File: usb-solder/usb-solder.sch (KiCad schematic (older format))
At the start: 303 parts, among them J1 USB_B_Micro, J10 USB_B_Micro, J11 USB_B_Micro, J12 USB_B_Micro, J13 USB_B_Micro, J14 USB_B_Micro, J15 USB_B_Micro, J16 USB_B_Micro, J17 USB_B_Micro, J18 USB_B_Micro, J19 USB_B_Micro, J2 USB_B_Micro, J20 USB_B_Micro, J21 USB_B_Micro, J22 USB_B_Micro, J23 USB_A, J24 Conn_01x02_Male, J25 Barrel_Jack_Switch, J26 USB_B_Micro, J27 Conn_01x07_Male, J3 USB_B_Micro, J4 USB_B_Micro, J5 USB_B_Micro, J6 USB_B_Micro, J7 USB_B_Micro, J8 USB_B_Micro, J9 USB_B_Micro, SW1 SW_SPDT, U1 555, U2 74HC164, U3 4072, U4 74AHC1G04, U5 AP1117-33

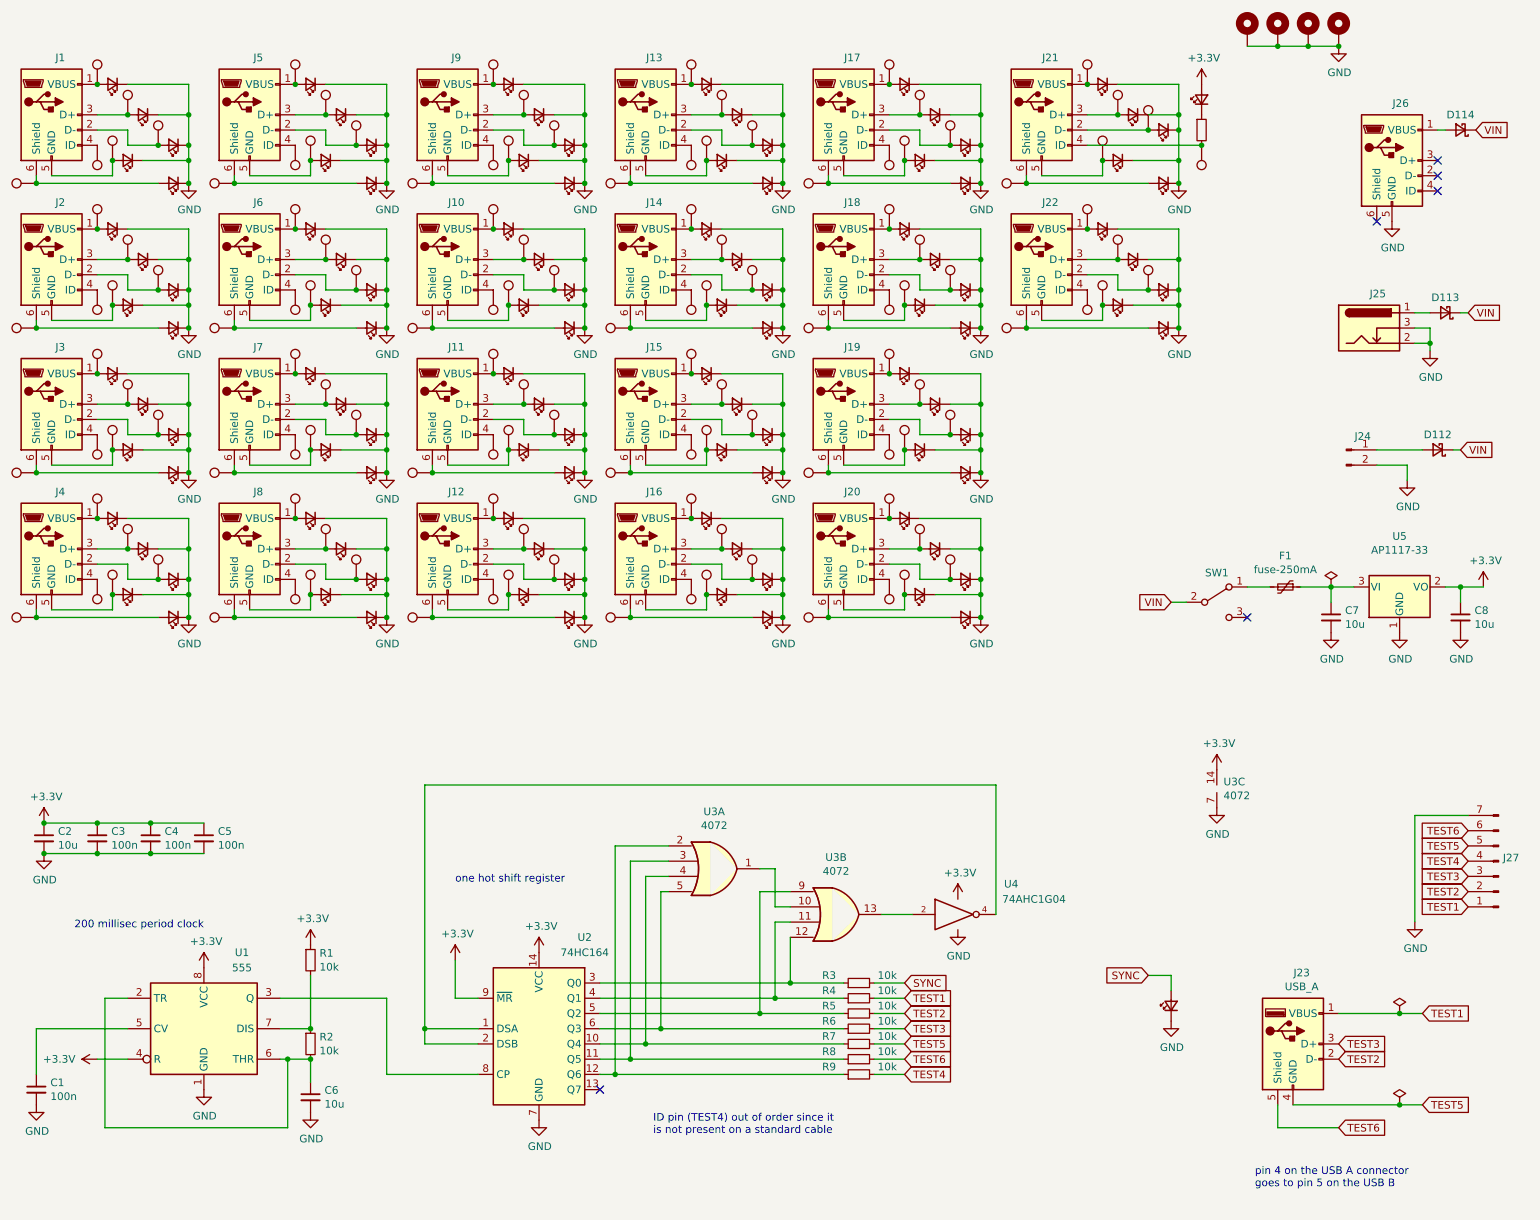
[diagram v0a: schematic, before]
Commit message: id
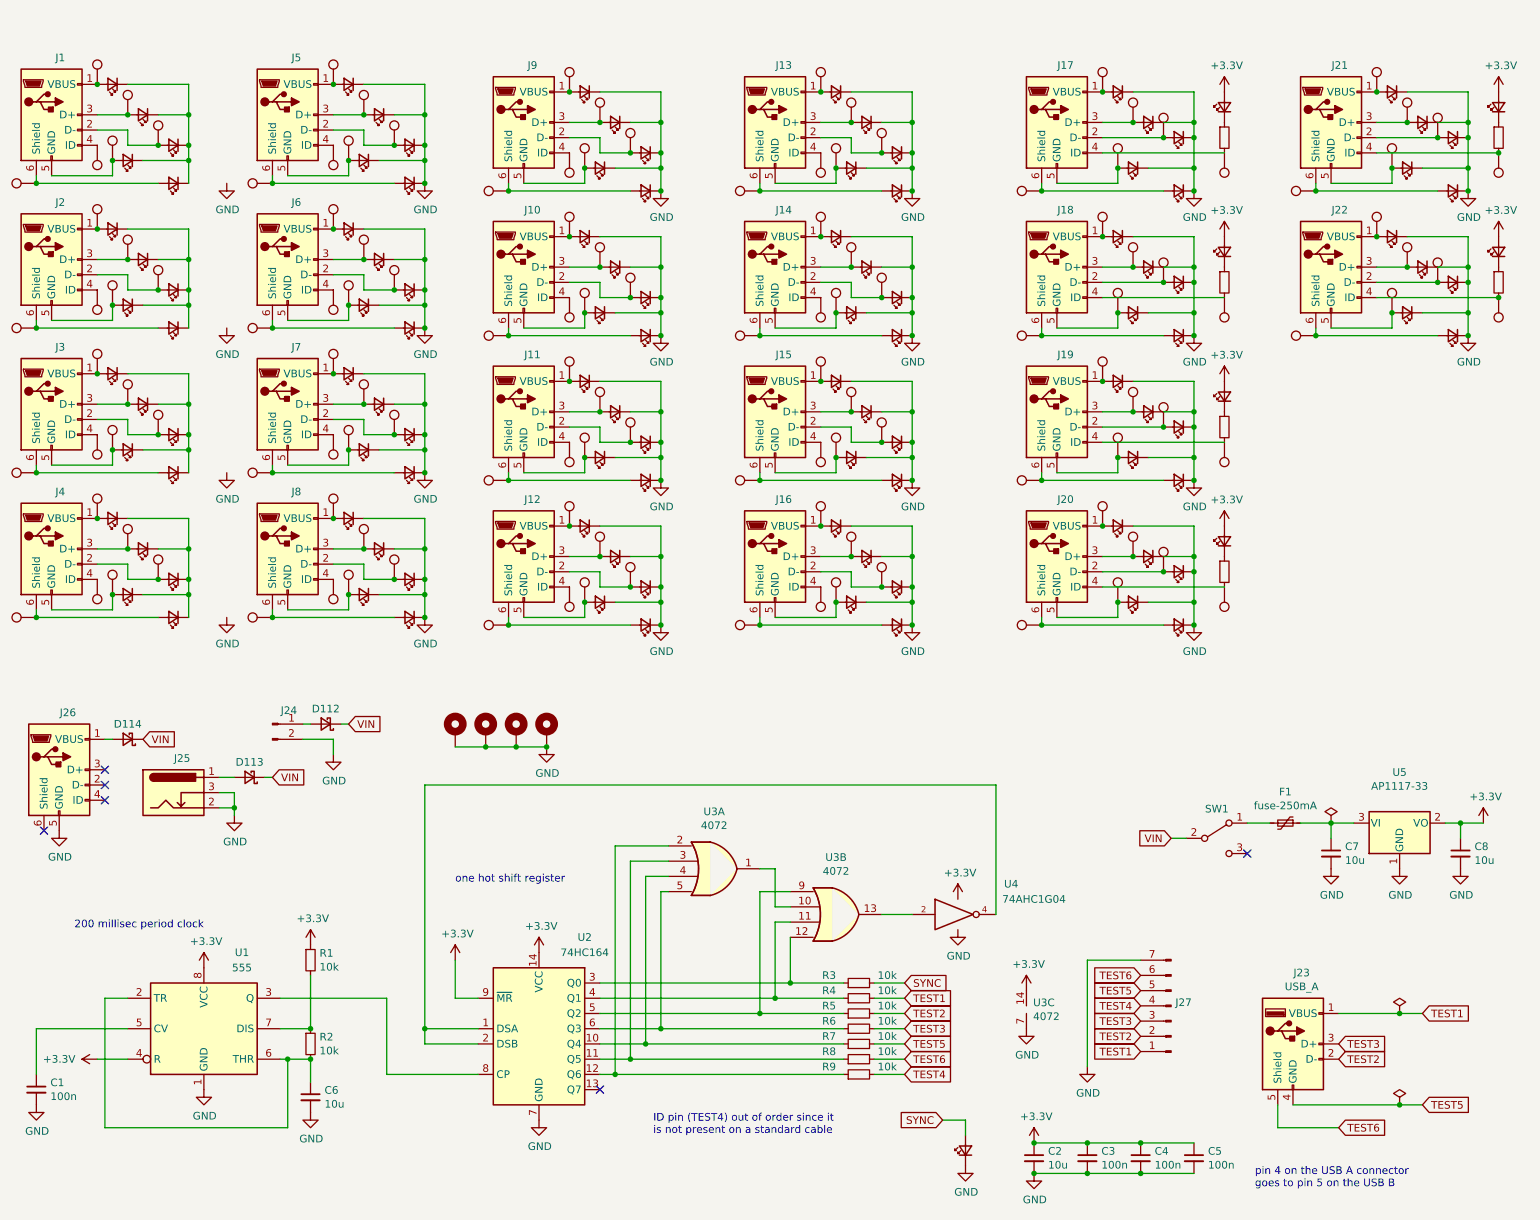
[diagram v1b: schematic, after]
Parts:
- added D116, D117, D118, D119, D120: ledred, LED_SMD:LED_0603_1608Metric, symbol pace:ledred
- added R11, R12, R13, R14, R15: 10k, Resistor_SMD:R_0402_1005Metric, symbol pace:10k
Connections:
- net +3V3: now also D116.2 (A), D117.2 (A), D118.2 (A), D119.2 (A), D120.2 (A)
- net GND: no longer D1.1 (K), D10.1 (K), D11.1 (K), D12.1 (K), D13.1 (K), D14.1 (K), D15.1 (K), D16.1 (K), D17.1 (K), D18.1 (K), D19.1 (K), D2.1 (K), D20.1 (K), D3.1 (K), D4.1 (K), D5.1 (K), D6.1 (K), D7.1 (K), D8.1 (K), D9.1 (K)
- net at J17.4 (ID), TP102.1: now also R11.2
- net at J18.4 (ID), TP104.1: now also R12.2
- net at J19.4 (ID), TP106.1: now also R13.2
- net at J20.4 (ID), TP108.1: now also R14.2
- net at J22.4 (ID), TP126.1: now also R15.2
- new net: D1.1 (K), D13.1 (K), D14.1 (K), D5.1 (K), D9.1 (K)
- new net: D10.1 (K), D15.1 (K), D16.1 (K), D2.1 (K), D6.1 (K)
- new net: D11.1 (K), D17.1 (K), D18.1 (K), D3.1 (K), D7.1 (K)
- new net: D12.1 (K), D19.1 (K), D20.1 (K), D4.1 (K), D8.1 (K)
- new net: D120.1 (K), R15.1
- new net: D116.1 (K), R11.1
- new net: D117.1 (K), R12.1
- new net: D118.1 (K), R13.1
- new net: D119.1 (K), R14.1
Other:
- moved on the sheet: C2, C3, C4, C5, C7, C8, D112, D113, D114, F1, J10, J11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

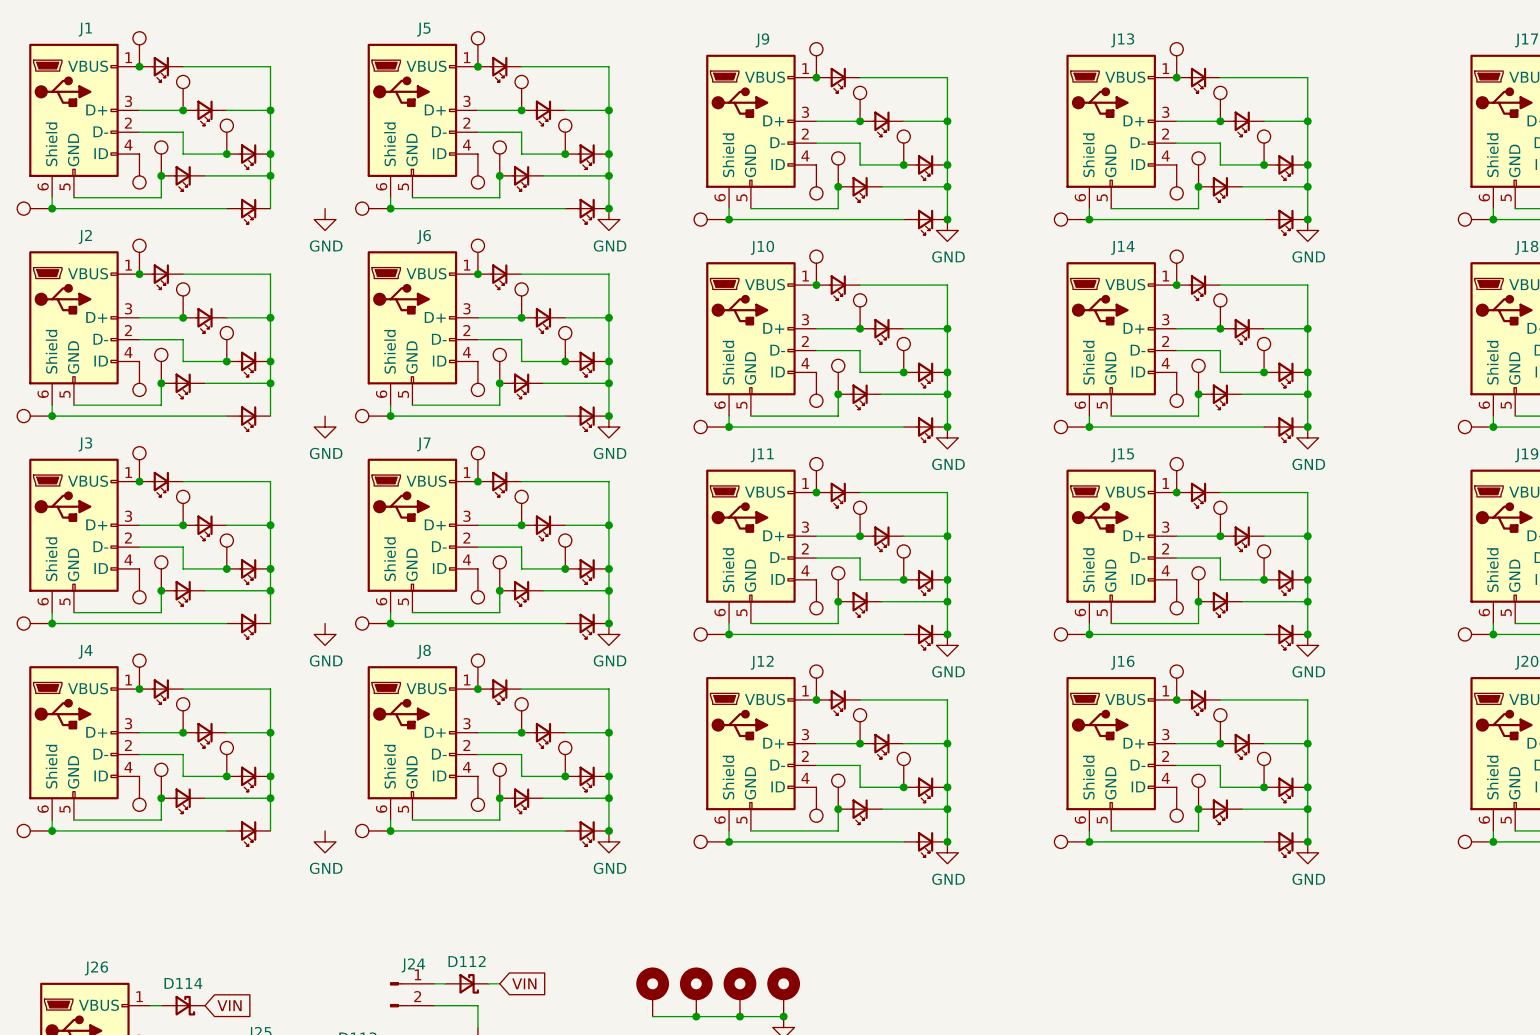
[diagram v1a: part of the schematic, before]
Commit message: id
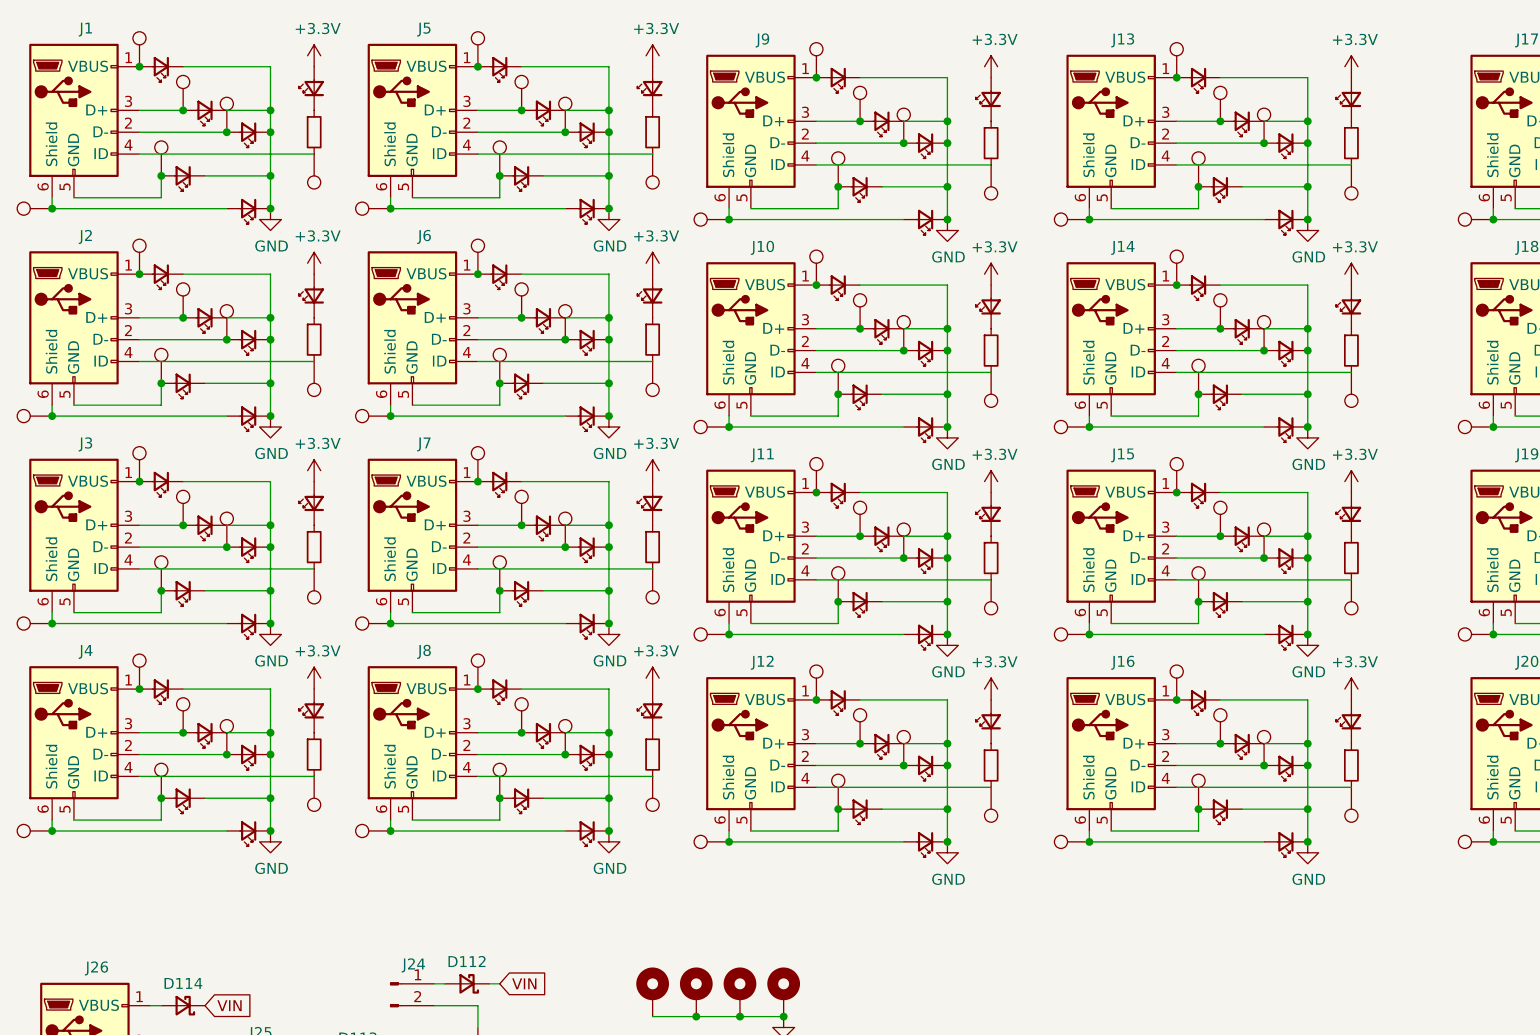
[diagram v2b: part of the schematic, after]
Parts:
- added D121, D122, D123, D124, D125, D126, D127, D128, D129, D130, D131, D132, D133, D134, D135, D136: ledred, LED_SMD:LED_0603_1608Metric, symbol pace:ledred
- added R16, R17, R18, R19, R20, R21, R22, R23, R24, R25, R26, R27, R28, R29, R30, R31: 10k, Resistor_SMD:R_0402_1005Metric, symbol pace:10k
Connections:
- net +3V3: now also D121.2 (A), D122.2 (A), D123.2 (A), D124.2 (A), D125.2 (A), D126.2 (A), D127.2 (A), D128.2 (A), D129.2 (A), D130.2 (A), D131.2 (A), D132.2 (A), D133.2 (A), D134.2 (A), D135.2 (A), D136.2 (A)
- net GND: now also D1.1 (K), D10.1 (K), D11.1 (K), D12.1 (K), D13.1 (K), D14.1 (K), D15.1 (K), D16.1 (K), D17.1 (K), D18.1 (K), D19.1 (K), D2.1 (K), D20.1 (K), D3.1 (K), D4.1 (K), D5.1 (K), D6.1 (K), D7.1 (K), D8.1 (K), D9.1 (K)
- net at J1.4 (ID), TP6.1: now also R16.2
- net at J2.4 (ID), TP8.1: now also R17.2
- net at J3.4 (ID), TP10.1: now also R18.2
- net at J4.4 (ID), TP12.1: now also R19.2
- net at J5.4 (ID), TP30.1: now also R20.2
- net at J6.4 (ID), TP32.1: now also R21.2
- net at J7.4 (ID), TP34.1: now also R22.2
- net at J8.4 (ID), TP36.1: now also R23.2
- net at J9.4 (ID), TP54.1: now also R24.2
- net at J10.4 (ID), TP56.1: now also R25.2
- net at J11.4 (ID), TP58.1: now also R26.2
- net at J12.4 (ID), TP60.1: now also R27.2
- net at J13.4 (ID), TP78.1: now also R28.2
- net at J14.4 (ID), TP80.1: now also R29.2
- net at J15.4 (ID), TP82.1: now also R30.2
- net at J16.4 (ID), TP84.1: now also R31.2
- new net: D133.1 (K), R28.1
- new net: D134.1 (K), R29.1
- new net: D135.1 (K), R30.1
- new net: D136.1 (K), R31.1
- new net: D132.1 (K), R27.1
- new net: D131.1 (K), R26.1
- new net: D130.1 (K), R25.1
- new net: D129.1 (K), R24.1
- new net: D125.1 (K), R20.1
- new net: D126.1 (K), R21.1
- new net: D127.1 (K), R22.1
- new net: D128.1 (K), R23.1
- new net: D124.1 (K), R19.1
- new net: D123.1 (K), R18.1
- new net: D122.1 (K), R17.1
- new net: D121.1 (K), R16.1
